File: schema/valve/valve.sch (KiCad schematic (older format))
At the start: 0 parts

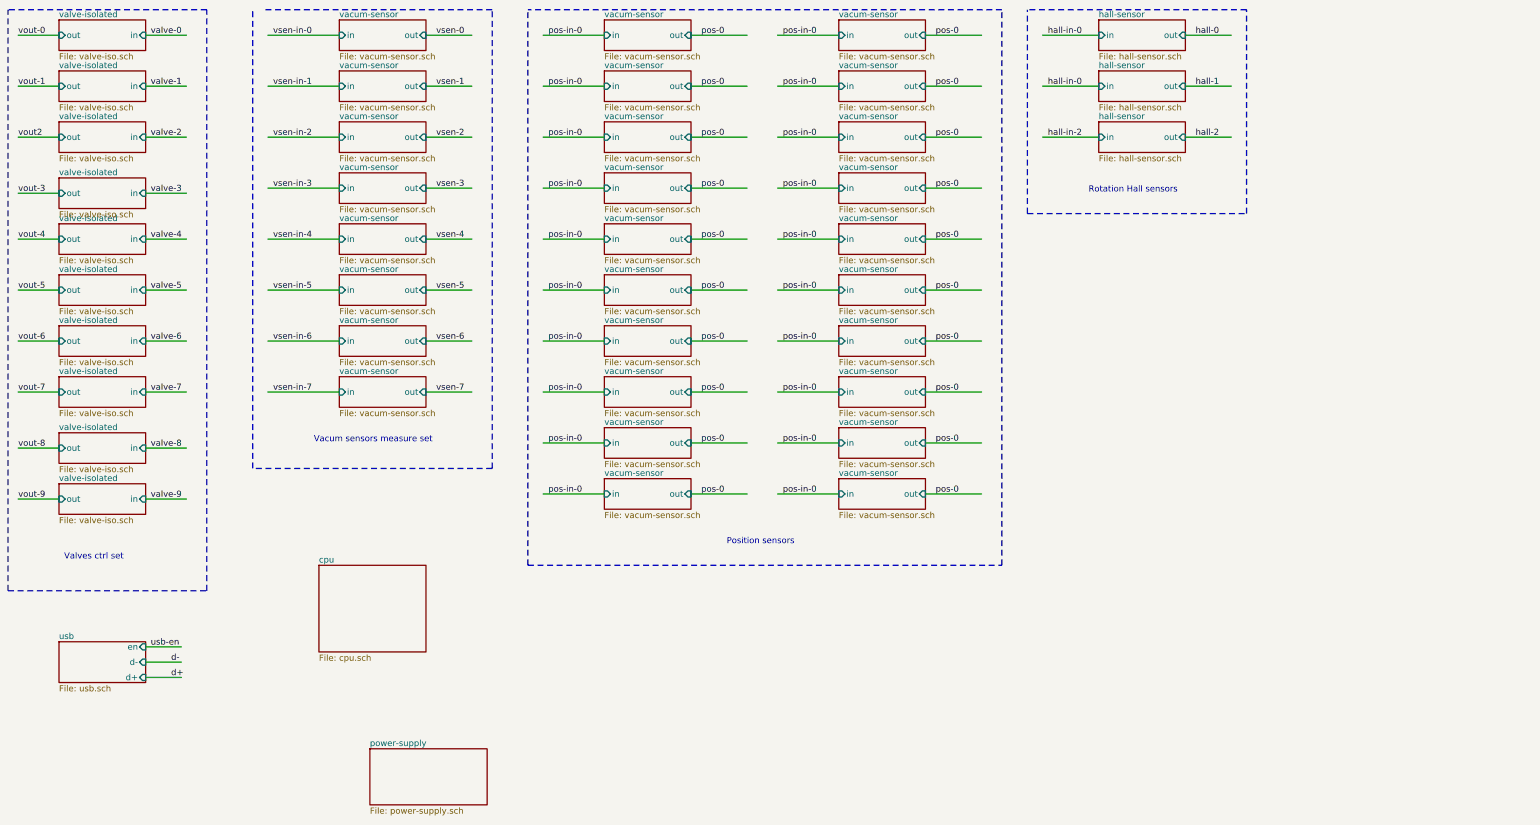
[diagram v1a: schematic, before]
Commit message: Signed-off-by: z80 <litedictteam@gmail.com>
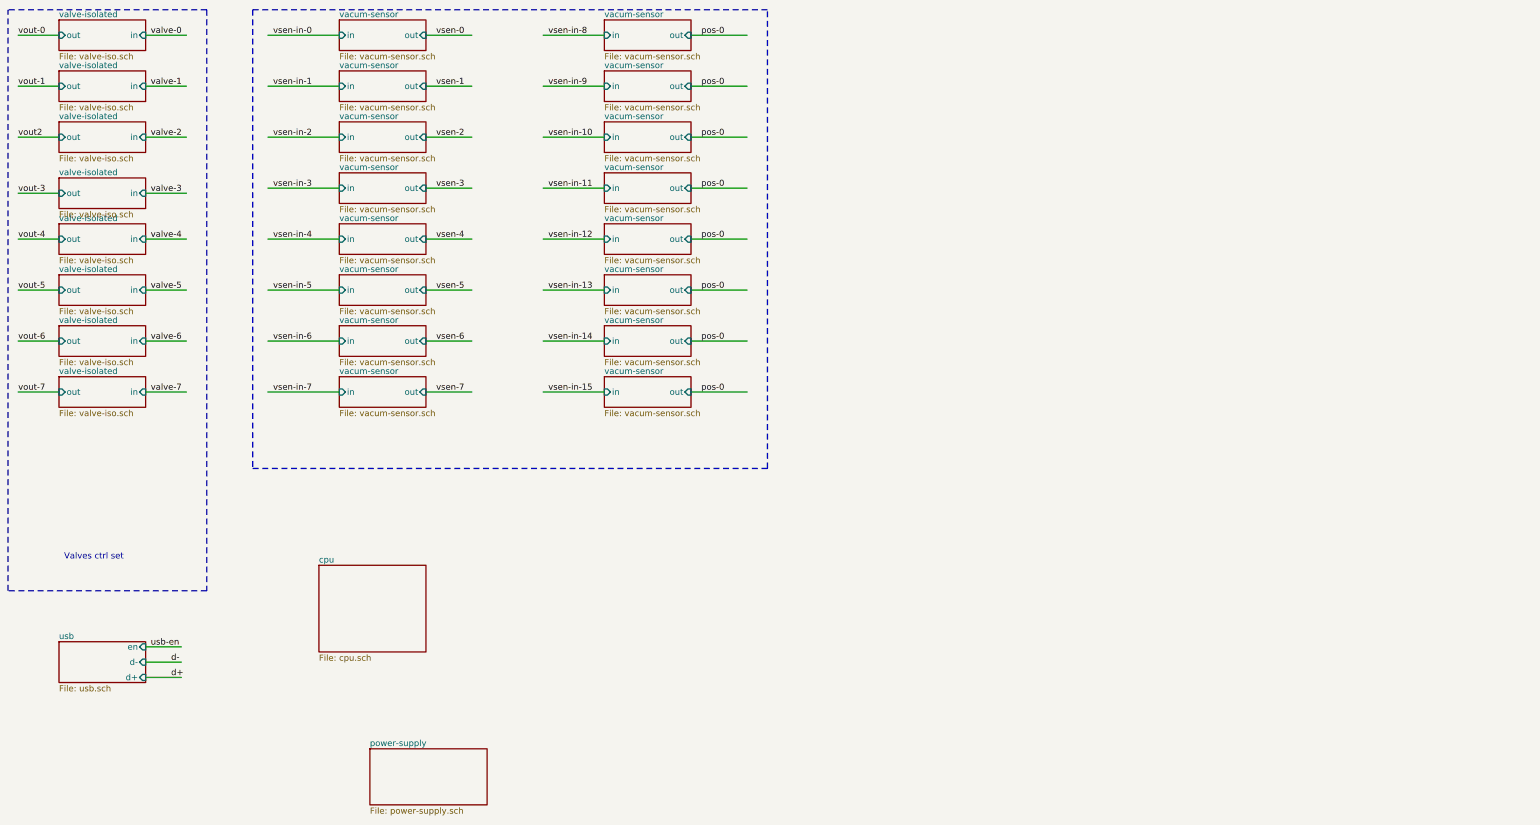
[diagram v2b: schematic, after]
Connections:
- net labels added: vsen-in-10, vsen-in-11, vsen-in-12, vsen-in-13, vsen-in-14, vsen-in-15, vsen-in-8, vsen-in-9
- net labels removed: hall-0, hall-1, hall-2, hall-in-0, hall-in-2, pos-in-0, valve-8, valve-9, vout-8, vout-9
- wire segments 85 -> 51
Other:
- note removed: "Position sensors"
- note removed: "Rotation Hall sensors"
- note removed: "Vacum sensors measure set"

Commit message: Schema, svg and png.
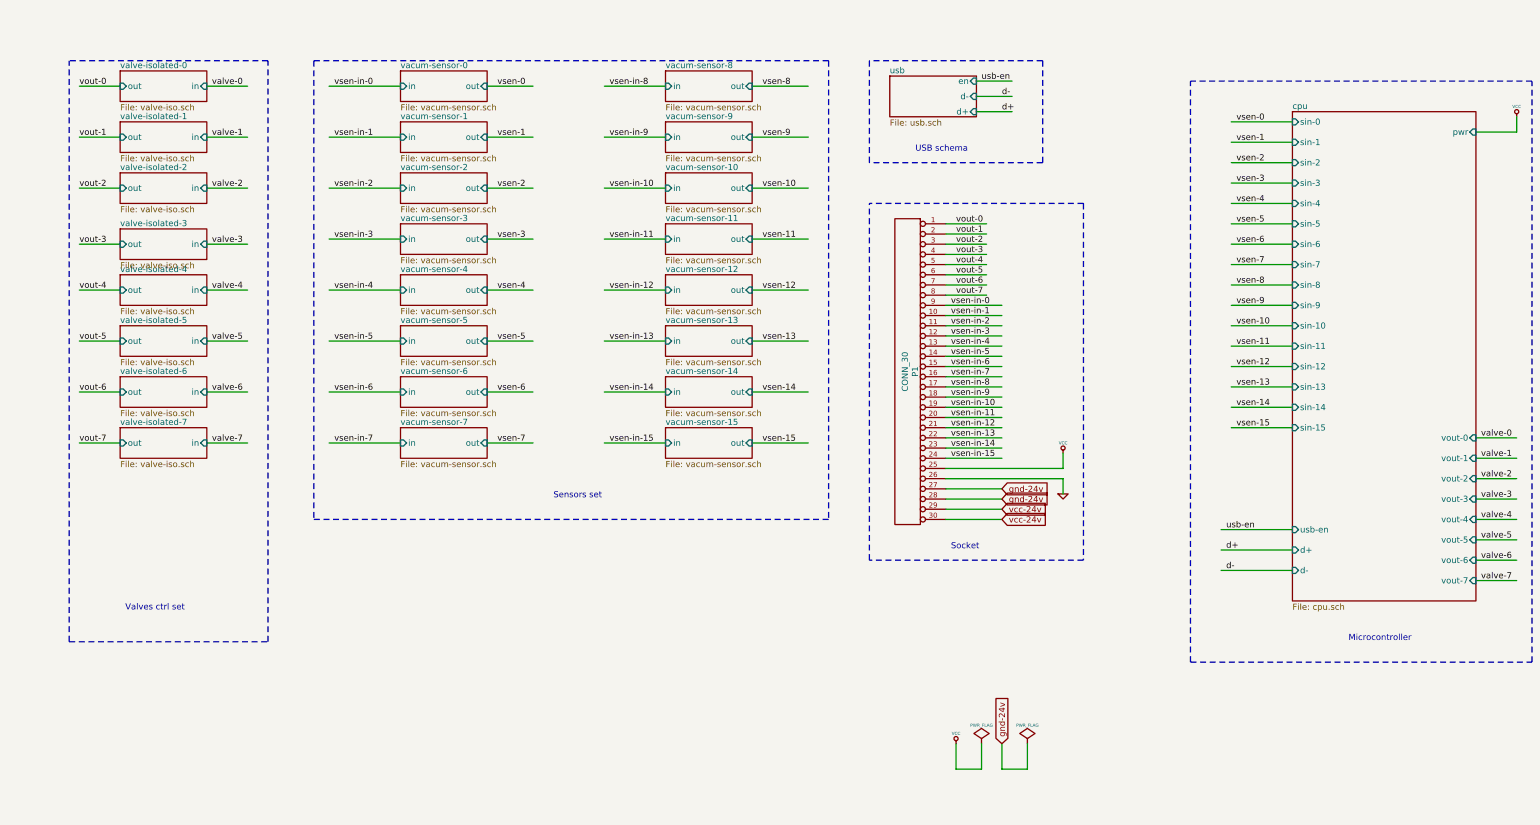
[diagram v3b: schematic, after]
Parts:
- added P1: CONN_30, symbol CONN_30
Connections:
- net labels added: GND, VCC, gnd-24v, vcc-24v, vout-2, vsen-10, vsen-11, vsen-12, vsen-13, vsen-14, vsen-15, vsen-8, vsen-9
- net labels removed: pos-0, vout2
- wire segments 51 -> 118
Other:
- note added: "Microcontroller"
- note added: "Sensors set"
- note added: "Socket"
- note added: "USB schema"
